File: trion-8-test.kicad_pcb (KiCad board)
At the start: 4 copper layers, 86 x 51.5 mm, 184 parts, among them J1 RJ45_Amphenol_RJMG1BD3B8K1ANR, J2 T8_JTAG, J3 T8_JTAG, J4 USB_C_Receptacle_USB2.0, J5 ETH GPIO, J6 FPGA GPIO, J7 FPGA_B3_GPIO, Q1 SSM3K37MFV, SW1 Reset, U1 MT48LC16M16A2P, U10 USB3343, U12 RT8096B, U2 dp83640, U6 RT8096B, U8 T8Q144xx, U9 AT25FF081A-SSHN-B, X1 ECS-2520MV-120-CM, X2 ECS-2520MV-120-CM, Y1 26MHz

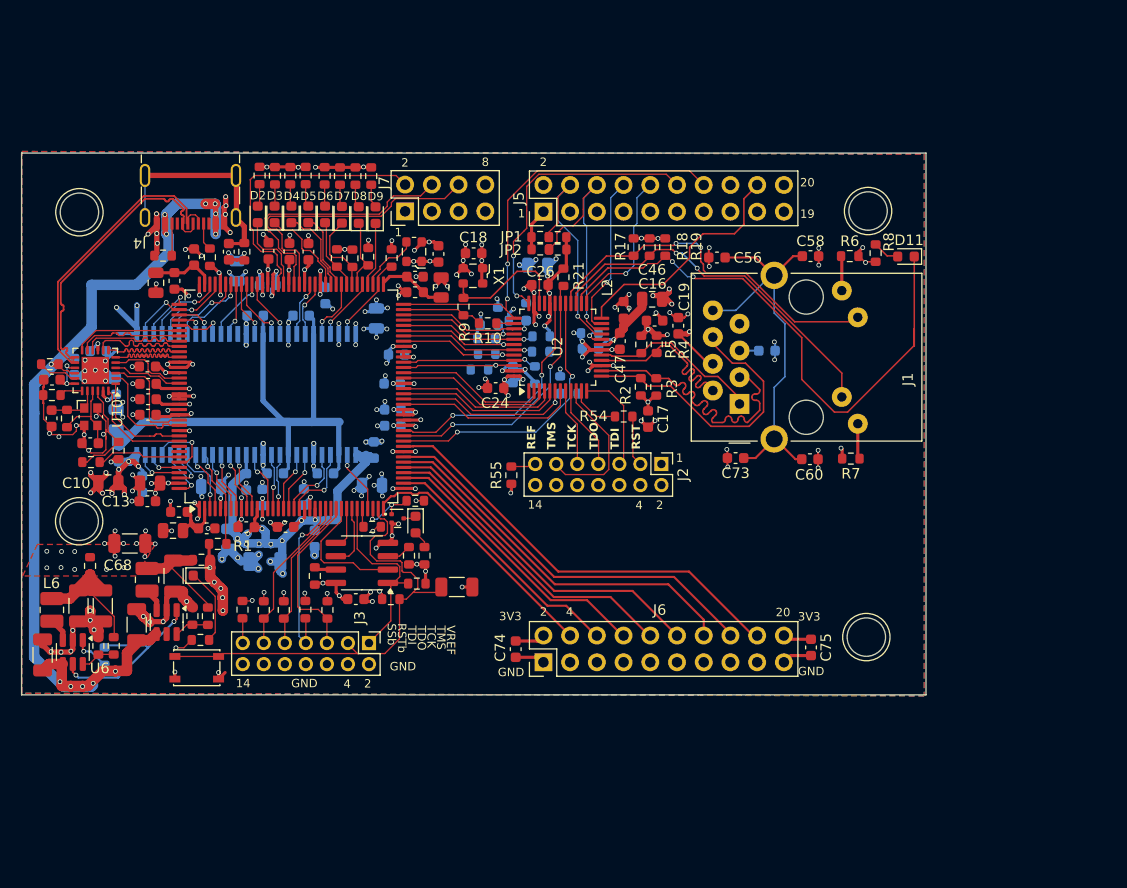
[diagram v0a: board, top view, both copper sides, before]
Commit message: Added GPS receiver; increased board size
including battery supply; made board bigger
and added edge connectors for ETH GPIO, PPS
and antenna.
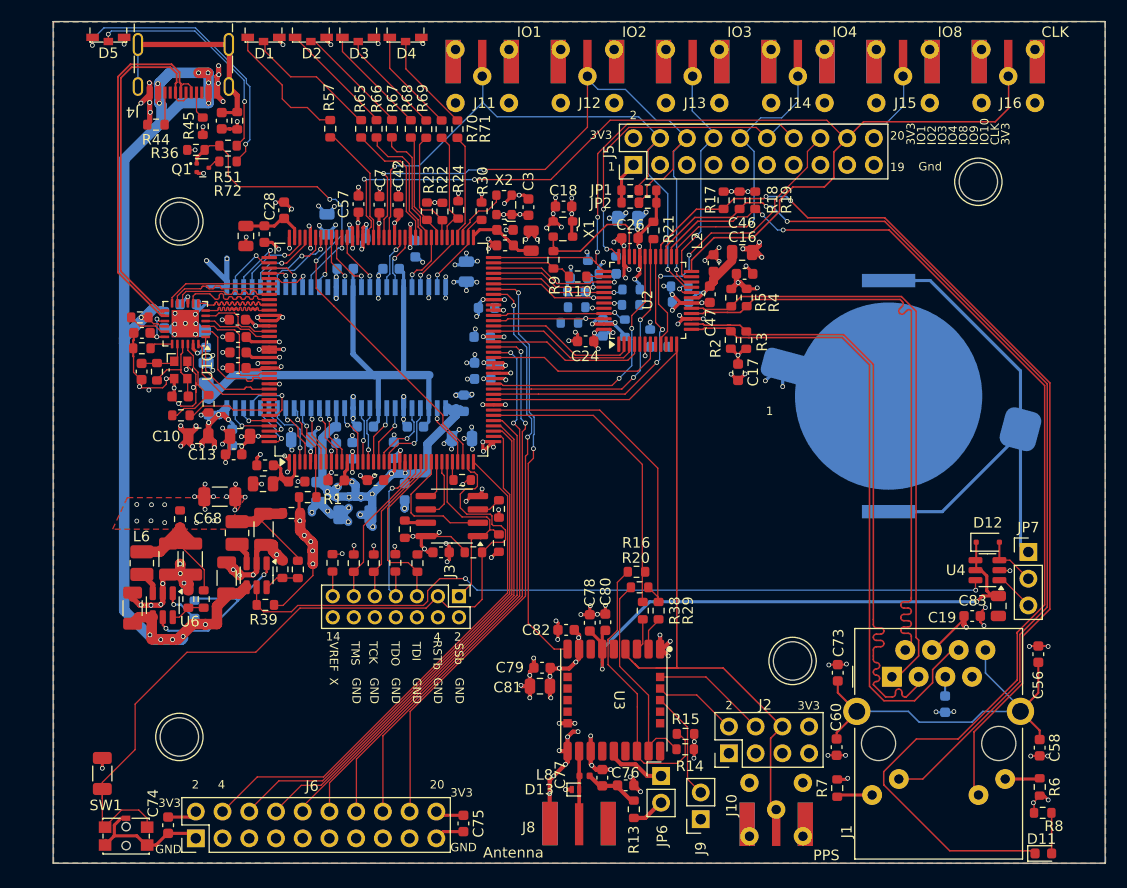
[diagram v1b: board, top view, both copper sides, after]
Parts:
- removed D10, D6, D7, D8, D9: LED, LED_SMD:LED_0603_1608Metric
- removed J7: FPGA_B3_GPIO, Connector_PinHeader_2.54mm:PinHeader_2x04_P2.54mm_Vertical
- removed R54: 0, Resistor_SMD:R_0603_1608Metric
- removed R55: 10k, Resistor_SMD:R_0603_1608Metric
- removed R64: 1k, Resistor_SMD:R_0603_1608Metric
- added BT1: Battery_Cell, battery:bh-3034-74-combined, B.Cu at (140.6, 95.8)
- added C76: 100n, Capacitor_SMD:C_0603_1608Metric, F.Cu at (114.4, 132.6)
- added C77: 50p, Capacitor_SMD:C_0603_1608Metric, F.Cu at (112.2, 131.9)
- added C78: 50p, Capacitor_SMD:C_0603_1608Metric, F.Cu at (111.0, 117.2)
- added C79: 100n, Capacitor_SMD:C_0603_1608Metric, F.Cu at (106.5, 121.4)
- added C80: 100n, Capacitor_SMD:C_0603_1608Metric, F.Cu at (112.5, 117.1)
- added C81: 4u7, Capacitor_SMD:C_0805_2012Metric, F.Cu at (106.3, 123.2)
- added C82: 50p, Capacitor_SMD:C_0603_1608Metric, F.Cu at (108.8, 117.8)
- added C83: 4u7, Capacitor_SMD:C_0805_2012Metric, F.Cu at (149.8, 115.5)
- added D12: D, Diode_SMD:D_SOD-323F, F.Cu at (148.8, 109.5)
- added D13: ~, Diode_SMD:D_SOD-882, F.Cu at (109.7, 133.0)
- added J10: PPS, proj_footprints:LEMO+SMA_molex_732515460, F.Cu at (128.7, 134.9)
- added J11: IO1, proj_footprints:LEMO+SMA_molex_732515460, F.Cu at (100.8, 65.2)
- added J12: IO2, proj_footprints:LEMO+SMA_molex_732515460, F.Cu at (110.8, 65.2)
- added J13: IO3, proj_footprints:LEMO+SMA_molex_732515460, F.Cu at (120.8, 65.2)
- added J14: IO4, proj_footprints:LEMO+SMA_molex_732515460, F.Cu at (130.8, 65.2)
- added J15: IO8, proj_footprints:LEMO+SMA_molex_732515460, F.Cu at (140.8, 65.2)
- added J16: CLK, proj_footprints:LEMO+SMA_molex_732515460, F.Cu at (150.8, 65.2)
- added J8: Antenna, proj_footprints:SMA Molex 732515460, F.Cu at (110.0, 138.3)
- added J9: Geofnc, Connector_PinSocket_2.54mm:PinSocket_1x02_P2.54mm_Vertical, F.Cu at (121.6, 135.8)
- added JP6: Jumper_2_Bridged, Connector_PinHeader_2.54mm:PinHeader_1x02_P2.54mm_Vertical, F.Cu at (117.8, 131.7)
- added JP7: Jumper_3_Bridged12, Connector_PinHeader_2.54mm:PinHeader_1x03_P2.54mm_Vertical, F.Cu at (152.7, 110.4)
- added L8: 100n, Inductor_SMD:L_0402_1005Metric, F.Cu at (110.5, 131.7)
- added R13: 210, Resistor_SMD:R_0603_1608Metric, F.Cu at (115.2, 134.9)
- added R14: 2k2, Resistor_SMD:R_0603_1608Metric, F.Cu at (120.1, 129.2)
- added R15: 2k2, Resistor_SMD:R_0603_1608Metric, F.Cu at (120.1, 127.7)
- added R16: 0, Resistor_SMD:R_0603_1608Metric, F.Cu at (115.5, 112.3)
- added R20: 0, Resistor_SMD:R_0603_1608Metric, F.Cu at (115.7, 113.8)
- added R29: 0, Resistor_SMD:R_0603_1608Metric, F.Cu at (117.5, 116.0)
- added R38: 0, Resistor_SMD:R_0603_1608Metric, F.Cu at (116.0, 116.0)
- added R39: 10k, Resistor_SMD:R_0603_1608Metric, F.Cu at (80.2, 115.5)
- added R51: 1k, Resistor_SMD:R_0603_1608Metric, F.Cu at (76.6, 71.8)
- added U3: LC76G, proj_footprints:lc76g, F.Cu at (113.3, 124.5)
- added U4: TS5A63157DBV, Package_TO_SOT_SMD:SOT-23-6, F.Cu at (148.8, 112.2)
- D1, D2, D3, D4, D5: value LED -> LED_Dual_RAG; footprint LED_SMD:LED_0603_1608Metric -> proj_footprints:LED_Wuerth_Sideview
- D11: value LED -> LED-GRN
- H1, H2, H3, H4: value Foot -> Foot FF-13-P3.5X5.5B
- J2: value T8_JTAG -> GPS_GPIO; footprint Connector_PinHeader_2.00mm:PinHeader_2x07_P2.00mm_Vertical -> Connector_PinHeader_2.54mm:PinHeader_2x04_P2.54mm_Vertical
- SW1: value Reset -> Reconfig; footprint Button_Switch_SMD:SW_SPST_PTS810 -> proj_footprints:SW_SPST_PTS810_and_PTS841
- U1: value MT48LC16M16A2P -> NDS36PT5-16ET
- U8: value T8Q144xx -> T20Q144xx
- X1, X2: value ECS-2520MV-120-CM -> ECS-2520MV-250-CM
- moved D11 58.2 mm to (154.1, 139.1), turned to 0 degrees
- moved R8 55.5 mm to (154.1, 135.2), turned to 0 degrees
- moved R6 53.6 mm to (153.8, 132.8), turned to -90 degrees
- moved C58 51.6 mm to (153.8, 129.0), turned to -90 degrees
- moved D1 50.8 mm to (80.0, 62.2), turned to 180 degrees
- moved C56 48.5 mm to (153.6, 120.1), turned to 90 degrees
- moved R72 41.9 mm to (76.6, 73.3), turned to 180 degrees
- moved R36 39.3 mm to (73.6, 72.2), turned to 0 degrees
- moved C19 39.3 mm to (147.4, 116.5), turned to 0 degrees
- moved Q1 38.1 mm to (74.2, 73.9)
- moved C45 38.1 mm to (64.7, 131.5), turned to 90 degrees
- moved C20 37.6 mm to (144.8, 124.9), turned to -90 degrees
- moved J6 37.0 mm to (73.6, 137.6)
- moved C75 37.0 mm to (99.0, 136.2)
- moved C74 37.0 mm to (70.9, 136.4)
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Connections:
- D1 pad 1: Net-(D1-K) -> Net-(D1-K1)
- D2 pad 1: LED0 -> Net-(D2-K1)
- D2 pad 2: Net-(D2-A) -> +3V3
- D3 pad 1: LED1 -> Net-(D3-K1)
- D3 pad 2: Net-(D3-A) -> +3V3
- D4 pad 1: LED2 -> Net-(D4-K1)
- D4 pad 2: Net-(D4-A) -> +3V3
- D5 pad 1: LED3 -> Net-(D5-K1)
- D5 pad 2: Net-(D5-A) -> +3V3
- J2 pad 1: unconnected-(J2-Pin_1-Pad1) -> GND
- J2 pad 2: GND -> Net-(J2-Pin_2)
- J2 pad 3: Net-(J2-Pin_3) -> GND
- J2 pad 4: GND -> Net-(J2-Pin_4)
- J2 pad 5: ETH0_TDI -> GND
- J2 pad 6: GND -> GPS_PPS
- J2 pad 7: ETH0_TDO -> GND
- J2 pad 8: GND -> +3V3
- J5 pad 16: GND -> ETH0_GPIO_10
- Q1 pad 3: Net-(D10-K) -> Net-(Q1-D)
- R57 pad 1: Net-(D2-A) -> LED0
- R57 pad 2: +3V3 -> Net-(D1-K2)
- R65 pad 1: Net-(D3-A) -> LED1
- R65 pad 2: +3V3 -> Net-(D1-K1)
- R66 pad 1: Net-(D4-A) -> LED2
- R66 pad 2: +3V3 -> Net-(D2-K2)
- R67 pad 1: Net-(D5-A) -> LED3
- R67 pad 2: +3V3 -> Net-(D2-K1)
- R68 pad 1: Net-(D6-A) -> LED4
- R68 pad 2: +3V3 -> Net-(D3-K2)
- R69 pad 1: Net-(D7-A) -> LED5
- R69 pad 2: +3V3 -> Net-(D3-K1)
- R70 pad 1: Net-(D8-A) -> LED6
- R70 pad 2: +3V3 -> Net-(D4-K2)
- R71 pad 1: Net-(D9-A) -> LED7
- R71 pad 2: +3V3 -> Net-(D4-K1)
- R72 pad 1: Net-(D10-A) -> Net-(D5-K2)
- R72 pad 2: +3V3 -> Net-(Q1-D)
- SW1 pad 1: Net-(J3-Pin_3) -> GND
- SW1 pad 2: GND -> Net-(J3-Pin_3)
- U12 pad 5: unconnected-(U12-PG-Pad5) -> POWER_GOOD
- U2 pad 10: ETH0_TMS -> unconnected-(U2-TMS-Pad10)
- U2 pad 11: ETH0_TRSTb -> unconnected-(U2-TRST#-Pad11)
- U2 pad 12: ETH0_TDI -> GPS_PPS
- U2 pad 5: ETH0_TXD_2 -> unconnected-(U2-TXD_2-Pad5)
- U2 pad 8: ETH0_TCK -> unconnected-(U2-TCK-Pad8)
- U2 pad 9: ETH0_TDO -> ETH0_GPIO_10
- U8 pad 42: FPGA_GPIO_5 -> UART_RX
- U8 pad 43: FPGA_GPIO_6 -> UART_TX
- U8 pad 45: FPGA_GPIO_7 -> GPS_PPS
- U8 pad 54: ETH0_TXD_3 -> FPGA_GPIO_5
- U8 pad 55: ETH0_TXD_2 -> FPGA_GPIO_6
- U8 pad 65: ETH0_RXD_2 -> FPGA_GPIO_7
- U8 pad 66: ETH0_RXD_3 -> GPS_RSTb
- U8 pad 89: FPGA_B3_IO_2 -> ETH0_GPIO_1
- U8 pad 90: FPGA_B3_IO_1 -> ETH0_GPIO_2
- U8 pad 93: FPGA_B3_IO_0 -> ETH0_CLK_OUT
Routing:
- net GPS_PPS: track 0.00 -> 80.9 mm
- net ETH0_CLK_OUT: track 22.8 -> 97.4 mm, vias 0 -> 2
- net POWER_GOOD: track 0.00 -> 73.7 mm, vias 0 -> 2
- net ETH0_LED_SPEED: track 35.1 -> 90.9 mm
- net Net-(D12-K): track 0.00 -> 54.6 mm, vias 0 -> 2
- net ETH0_LED_LINK: track 34.8 -> 89.1 mm
- net ETH0_LED_ACT: track 55.2 -> 108.4 mm
- net Net-(BT1-+): track 0.00 -> 50.0 mm
- net ETH0_GPIO_2: track 23.8 -> 67.5 mm, vias 1 -> 3
- net Net-(Q1-G): track 5.93 -> 49.6 mm
- net ETH0_TDP: track 16.4 -> 59.5 mm
- net ETH0_TDN: track 18.2 -> 60.1 mm
- net GND: track 249.3 -> 289.6 mm, vias 176 -> 206
- net GPS_RSTb: track 0.00 -> 39.6 mm, vias 0 -> 2
- net ETH0_GPIO_1: track 22.6 -> 61.5 mm, vias 1 -> 2
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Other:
- board size 86 x 51.5 mm -> 100 x 80 mm
- board text added: "CLK"
- board text added: "Gnd"
- board text added: "IO1"
- board text added: "IO10"
- board text added: "IO2"
- board text added: "IO3"
- board text added: "IO4"
- board text added: "IO8"
- board text added: "IO9"
- board text added: "Tic-Nic V2.0"
- board text added: "X"
- board text removed: "8"
- board text removed: "REF"
- board text removed: "RST"
- board text removed: "Trion-SDRAM-Test V2.0"
